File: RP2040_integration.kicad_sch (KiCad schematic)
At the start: 37 parts, among them J1 USB_B_Micro, J15 SWD, J2 Conn_01x02, U1 NCP1117-3.3_SOT223, U2 W25Q128JVS, U3 RP2040, Y1 ABM8-272-T3

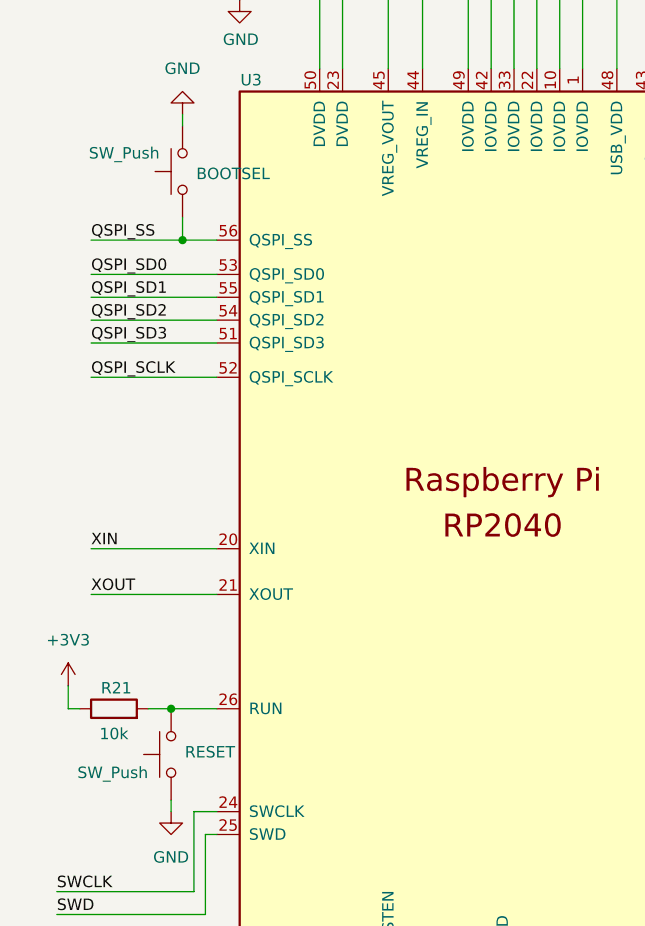
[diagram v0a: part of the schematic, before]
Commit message: last modifications
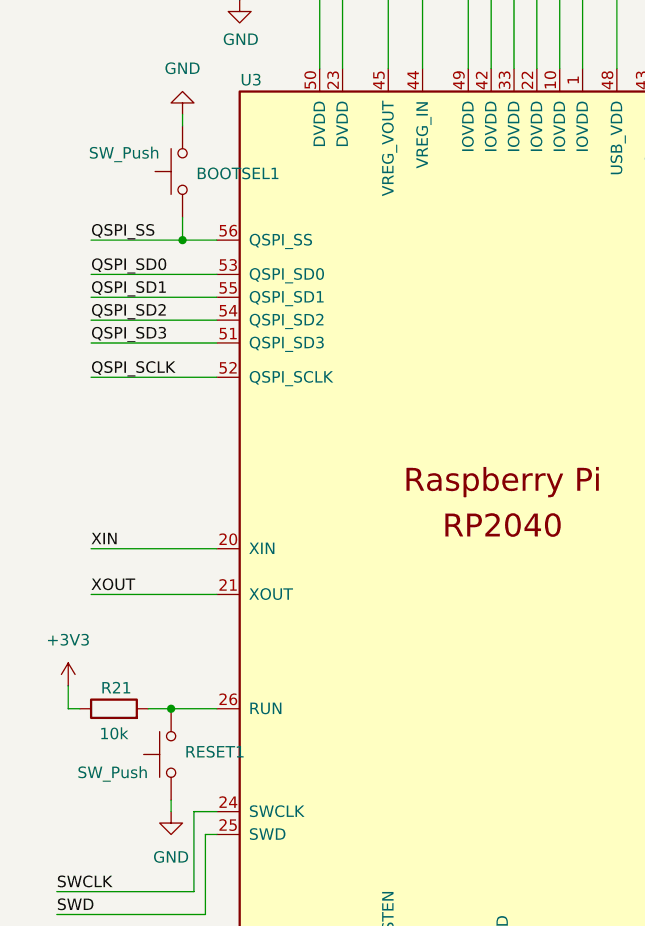
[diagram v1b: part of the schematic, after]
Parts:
- renumbered BOOTSEL to BOOTSEL1, RESET to RESET1
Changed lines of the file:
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@@
 		(on_board yes)
 		(dnp no)
-		(property "Reference" "BOOTSEL"
+		(property "Reference" "BOOTSEL1"
 			(at 66.294 113.284 90)
 			(effects
@@
 			(project "Valvotron8000Pro"
 				(path "/e783bbdf-2a7f-40b9-9fb7-b62785862857/e081148b-fef9-4fa9-8f75-119abd10d809"
-					(reference "BOOTSEL")
+					(reference "BOOTSEL1")
 					(unit 1)
 				)
@@
 		(on_board yes)
 		(dnp no)
-		(property "Reference" "RESET"
+		(property "Reference" "RESET1"
 			(at 65.024 177.546 90)
 			(effects
@@
 			(project ""
 				(path "/e783bbdf-2a7f-40b9-9fb7-b62785862857/e081148b-fef9-4fa9-8f75-119abd10d809"
-					(reference "RESET")
-					(unit 1)
-				)
+					(reference "RESET1")
+					(unit 1)
+				)

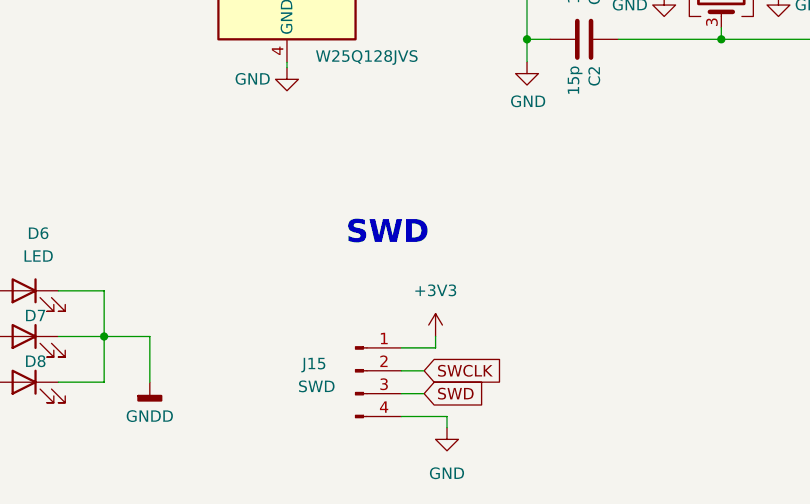
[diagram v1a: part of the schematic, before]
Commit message: Dernières modifs
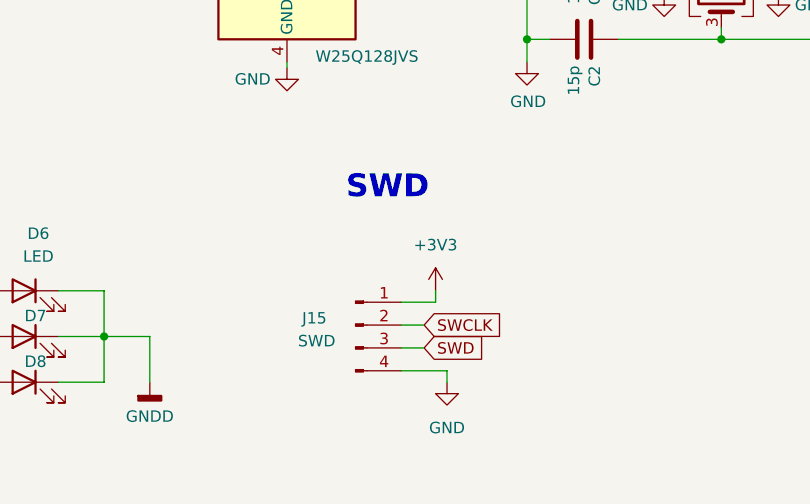
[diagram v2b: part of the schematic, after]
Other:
- moved on the sheet: J15
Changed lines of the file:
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@@
 	(text "SWD"
 		(exclude_from_sim no)
-		(at 262.636 212.09 0)
+		(at 262.636 207.01 0)
 		(effects
 			(font
@@
 	(wire
 		(pts
-			(xy 269.24 232.41) (xy 269.24 233.68)
+			(xy 269.24 227.33) (xy 269.24 228.6)
 		)
 		(stroke
@@
 	(wire
 		(pts
-			(xy 264.16 227.33) (xy 266.7 227.33)
+			(xy 264.16 222.25) (xy 266.7 222.25)
 		)
 		(stroke
@@
 	(wire
 		(pts
-			(xy 264.16 224.79) (xy 267.97 224.79)
+			(xy 264.16 219.71) (xy 267.97 219.71)
 		)
 		(stroke
@@
 	(wire
 		(pts
-			(xy 264.16 229.87) (xy 266.7 229.87)
+			(xy 264.16 224.79) (xy 266.7 224.79)
 		)
 		(stroke
@@
 	(wire
 		(pts
-			(xy 264.16 232.41) (xy 269.24 232.41)
+			(xy 264.16 227.33) (xy 269.24 227.33)
 		)
 		(stroke
@@
 	(wire
 		(pts
-			(xy 267.97 223.52) (xy 267.97 224.79)
+			(xy 267.97 218.44) (xy 267.97 219.71)
 		)
 		(stroke
@@
 	(global_label "SWD"
 		(shape input)
-		(at 266.7 229.87 0)
+		(at 266.7 224.79 0)
 		(fields_autoplaced yes)
 		(effects
@@
 		)
 		(property "Intersheetrefs" "${INTERSHEET_REFS}"
-			(at 273.6161 229.87 0)
+			(at 273.6161 224.79 0)
 			(effects
 				(font
@@
 	(global_label "SWCLK"
 		(shape input)
-		(at 266.7 227.33 0)
+		(at 266.7 222.25 0)
 		(fields_autoplaced yes)
 		(effects
@@
 		)
 		(property "Intersheetrefs" "${INTERSHEET_REFS}"
-			(at 275.9142 227.33 0)
+			(at 275.9142 222.25 0)
 			(effects
 				(font
@@
 		(polyline
 			(pts
-				(xy 248.92 214.63) (xy 276.86 214.63) (xy 278.13 215.9) (xy 278.13 238.76) (xy 276.86 240.03) (xy 252.73 240.03)
-				(xy 247.65 234.95) (xy 247.65 215.9)
+				(xy 248.92 209.55) (xy 276.86 209.55) (xy 278.13 210.82) (xy 278.13 233.68) (xy 276.86 234.95) (xy 252.73 234.95)
+				(xy 247.65 229.87) (xy 247.65 210.82)
 			)
 			(stroke
@@
 	(symbol
 		(lib_id "Connector:Conn_01x04_Pin")
-		(at 259.08 227.33 0)
+		(at 259.08 222.25 0)
 		(unit 1)
 		(exclude_from_sim no)
@@
 		(dnp no)
 		(property "Reference" "J15"
-			(at 254.508 226.568 0)
+			(at 254.508 221.488 0)
 			(effects
 				(font
@@
 		)
 		(property "Value" "SWD"
-			(at 254.762 229.108 0)
+			(at 254.762 224.028 0)
 			(effects
 				(font
@@
 		)
 		(property "Footprint" "Connector_PinHeader_2.54mm:PinHeader_1x04_P2.54mm_Vertical"
-			(at 259.08 227.33 0)
+			(at 259.08 222.25 0)
 			(effects
 				(font
@@
 		)
 		(property "Datasheet" "~"
-			(at 259.08 227.33 0)
+			(at 259.08 222.25 0)
 			(effects
 				(font
@@
 		)
 		(property "Description" "Generic connector, single row, 01x04, script generated"
-			(at 259.08 227.33 0)
+			(at 259.08 222.25 0)
 			(effects
 				(font
@@
 		(lib_name "+3V3_2")
 		(lib_id "power:+3V3")
-		(at 267.97 223.52 0)
+		(at 267.97 218.44 0)
 		(unit 1)
 		(exclude_from_sim no)
@@
 		(fields_autoplaced yes)
 		(property "Reference" "#PWR0103"
-			(at 267.97 227.33 0)
+			(at 267.97 222.25 0)
 			(effects
 				(font
@@
 		)
 		(property "Value" "+3V3"
-			(at 267.97 218.44 0)
+			(at 267.97 213.36 0)
 			(effects
 				(font
@@
 		)
 		(property "Footprint" ""
-			(at 267.97 223.52 0)
+			(at 267.97 218.44 0)
 			(effects
 				(font
@@
 		)
 		(property "Datasheet" ""
-			(at 267.97 223.52 0)
+			(at 267.97 218.44 0)
 			(effects
 				(font
@@
 		)
 		(property "Description" "Power symbol creates a global label with name \"+3V3\""
-			(at 267.97 223.52 0)
+			(at 267.97 218.44 0)
 			(effects
 				(font
@@
 	(symbol
 		(lib_id "DPR_devices:GND")
-		(at 269.24 233.68 0)
+		(at 269.24 228.6 0)
 		(unit 1)
 		(exclude_from_sim no)
@@
 		(fields_autoplaced yes)
 		(property "Reference" "#PWR0104"
-			(at 269.24 240.03 0)
+			(at 269.24 234.95 0)
 			(effects
 				(font
@@
 		)
 		(property "Value" "GND"
-			(at 269.24 238.76 0)
+			(at 269.24 233.68 0)
 			(effects
 				(font
@@
 		)
 		(property "Footprint" ""
-			(at 269.24 233.68 0)
+			(at 269.24 228.6 0)
 			(effects
 				(font
@@
 		)
 		(property "Datasheet" ""
-			(at 269.24 233.68 0)
+			(at 269.24 228.6 0)
 			(effects
 				(font
@@
 		)
 		(property "Description" "Power symbol creates a global label with name \"GND\" , ground"
-			(at 269.24 233.68 0)
+			(at 269.24 228.6 0)
 			(effects
 				(font
